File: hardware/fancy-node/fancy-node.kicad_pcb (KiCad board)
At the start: 2 copper layers, 59.2 x 37 mm, 56 parts, among them J1 Conn_01x06, J2 Conn_01x02, J3 Conn_01x04, J4 USB_B_Micro, J5 Conn_01x03, SW1 SW_Push, SW2 SW_Push, SW3 SW_DPDT_x2, SW4 SW_Push, U1 CH340C, U2 STM32G030C8T6, U3 WS2812b, U5 HT75xx-1-SOT89, U6 RFM69CW-915MHZ, U7 TP4056

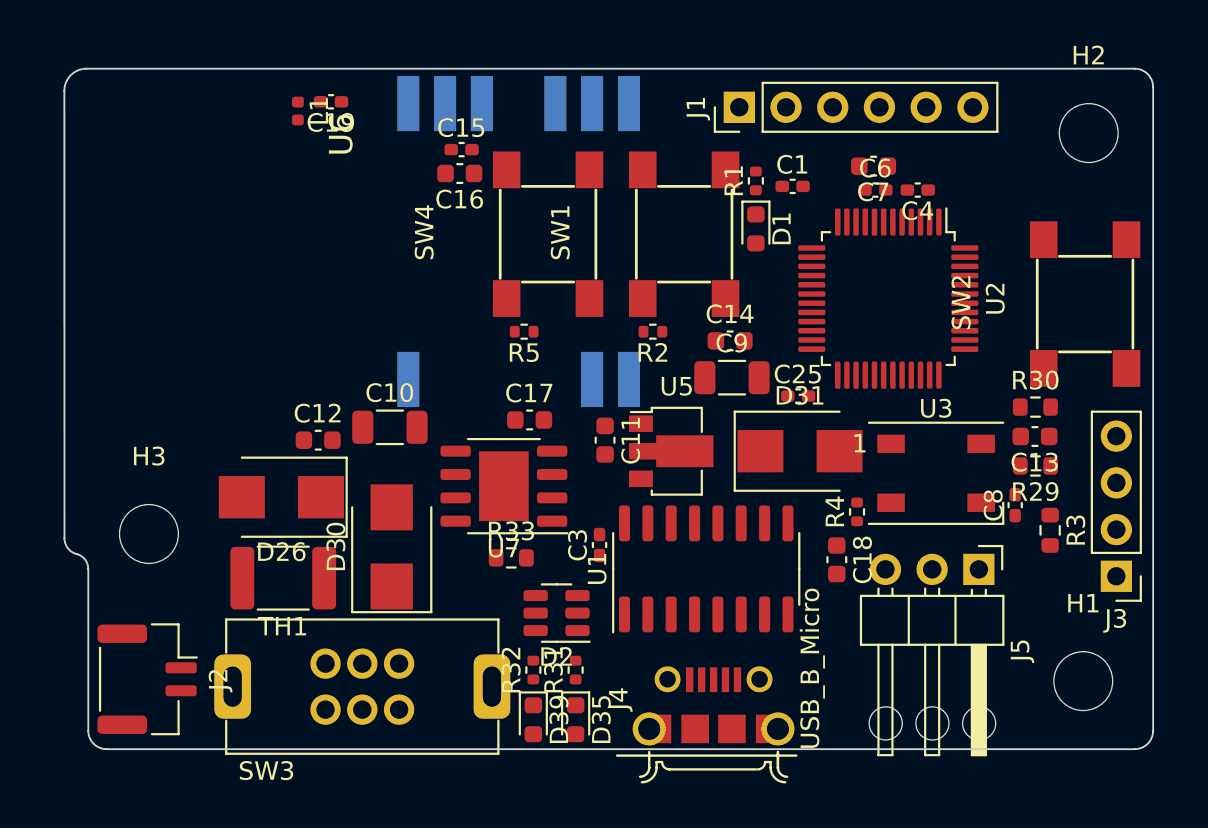
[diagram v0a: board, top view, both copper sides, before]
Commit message: fancy-node v1.0
Change-Id: I2dc287329bd6c7a9f578761cfc67db086f282b4b
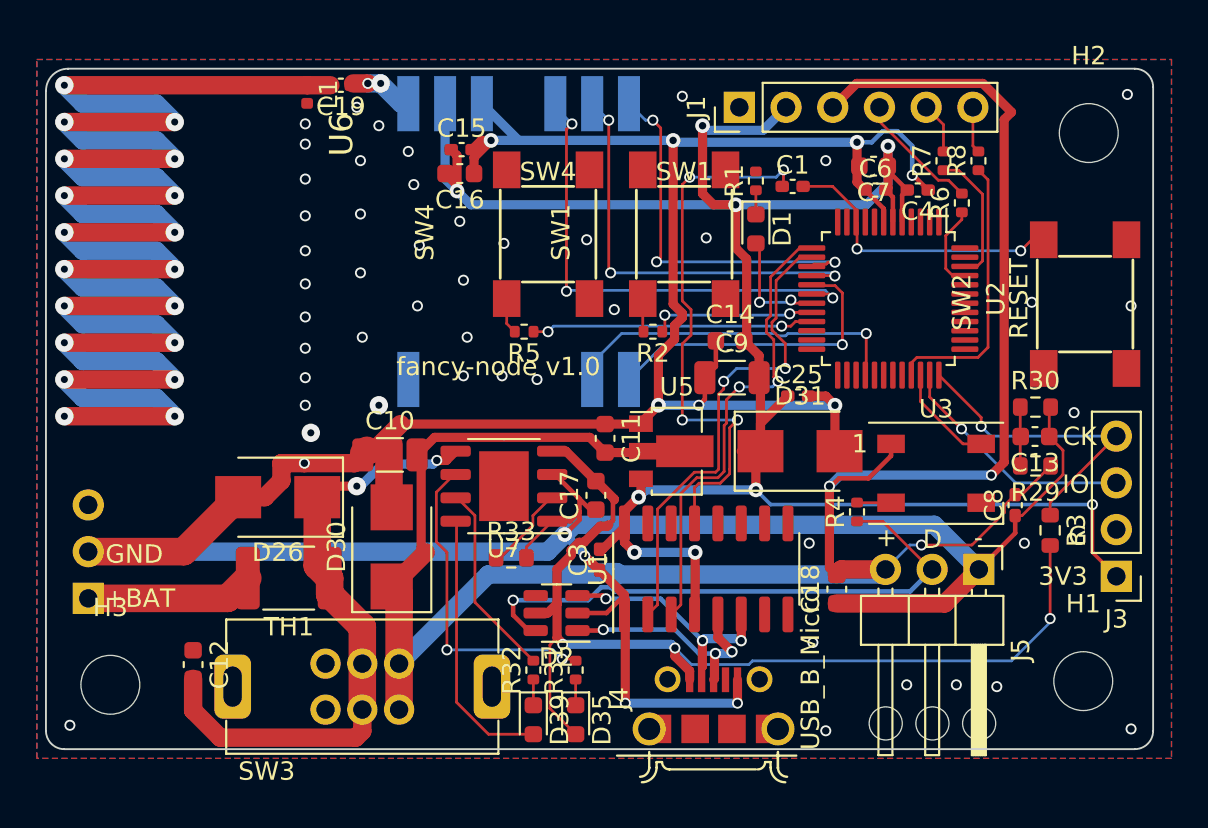
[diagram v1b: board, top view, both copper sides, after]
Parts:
- added R6: 1k, Resistor_SMD:R_0402_1005Metric, F.Cu at (76.6, 71.8)
- added R7: 1k, Resistor_SMD:R_0402_1005Metric, F.Cu at (75.6, 69.5)
- added R8: 1k, Resistor_SMD:R_0402_1005Metric, F.Cu at (77.5, 69.5)
- J2: value Conn_01x02 -> Conn_01x03; footprint Connector_JST:JST_GH_SM02B-GHS-TB_1x02-1MP_P1.25mm_Horizontal -> Homebrew:MiniPV_78208-X03XXX_1x03_P2.54mm_Polarized_Horizontal; moved to B.Cu
- moved C12 14.0 mm to (34.8, 96.9), turned to -90 degrees
- moved H3 8.46 mm to (30.3, 98.0)
- moved C17 5.46 mm to (56.7, 87.7), turned to 90 degrees
- moved J2 5.44 mm to (29.1, 93.3), turned to 0 degrees
- moved C18 1.60 mm to (69.8, 92.8), turned to 90 degrees
- moved C10 1.50 mm to (45.5, 85.5)
- moved C19 1.05 mm to (42.8, 65.4)
- moved L1 1.03 mm to (41.0, 65.9)
- moved C3 0.80 mm to (56.9, 91.2)
- moved TH1 0.30 mm to (40.0, 92.2)
- moved D26 0.20 mm to (39.4, 87.8)
- moved C11 0.10 mm to (57.2, 84.6)
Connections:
- J1 pad 4: /AUX0 -> Net-(J1-Pad4)
- J1 pad 5: /AUX1 -> Net-(J1-Pad5)
- J1 pad 6: /AUX2 -> Net-(J1-Pad6)
- J2 pad 1: GND -> Net-(TH1-Pad2)
- J2 pad 2: Net-(TH1-Pad2) -> GND
- U2 pad 29: /AUX0 -> unconnected-(U2-Pad29)
- U2 pad 32: /AUX1 -> unconnected-(U2-Pad32)
- U2 pad 45: unconnected-(U2-Pad45) -> /AUX0
- U2 pad 46: unconnected-(U2-Pad46) -> /AUX1
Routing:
- net GND: track 0.00 -> 209.6 mm, vias 0 -> 58
- net /ANTENNA: track 0.00 -> 129.9 mm, vias 0 -> 19
- net +BATT: track 0.00 -> 120.8 mm, vias 0 -> 3
- net VCC: track 0.00 -> 118.2 mm, vias 0 -> 9
- net VBUS: track 0.00 -> 55.8 mm, vias 0 -> 3
- net /BATT_DIRECT: track 0.00 -> 34.1 mm, vias 0 -> 2
- net /EXTERNAL_LED: track 0.00 -> 31.2 mm, vias 0 -> 1
- net /~{DTR}: track 0.00 -> 30.2 mm, vias 0 -> 4
- net /MOSI: track 0.00 -> 26.6 mm, vias 0 -> 3
- net /USART_RX: track 0.00 -> 26.3 mm, vias 0 -> 2
- net /USART_TX: track 0.00 -> 25.7 mm, vias 0 -> 2
- net /SCK: track 0.00 -> 23.2 mm, vias 0 -> 3
- net /NSS: track 0.00 -> 20.7 mm, vias 0 -> 3
- net /DIO0: track 0.00 -> 18.9 mm, vias 0 -> 1
- net /~{STDBY}: track 0.00 -> 17.5 mm, vias 0 -> 2
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- added copper zone on B.Cu, net GND
- added copper zone on F.Cu, net GND
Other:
- board size 59.2 x 37 mm -> 60.2 x 37 mm
- board text added: "+"
- board text added: "+BAT"
- board text added: "-"
- board text added: "3V3"
- board text added: "AUX0"
- board text added: "AUX1"
- board text added: "AUX2"
- board text added: "CK"
- board text added: "D"
- board text added: "G"
- board text added: "GND"
- board text added: "IO"
- board text added: "OFF"
- board text added: "ON"
- board text added: "RESET"
- board text added: "SW1"
- board text added: "SW4"
- board text added: "VCC"
- board text added: "fancy-node v1.0"
